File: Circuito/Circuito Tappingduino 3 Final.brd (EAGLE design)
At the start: 90.5 x 69 mm, 67 parts, among them IC1 LM324N

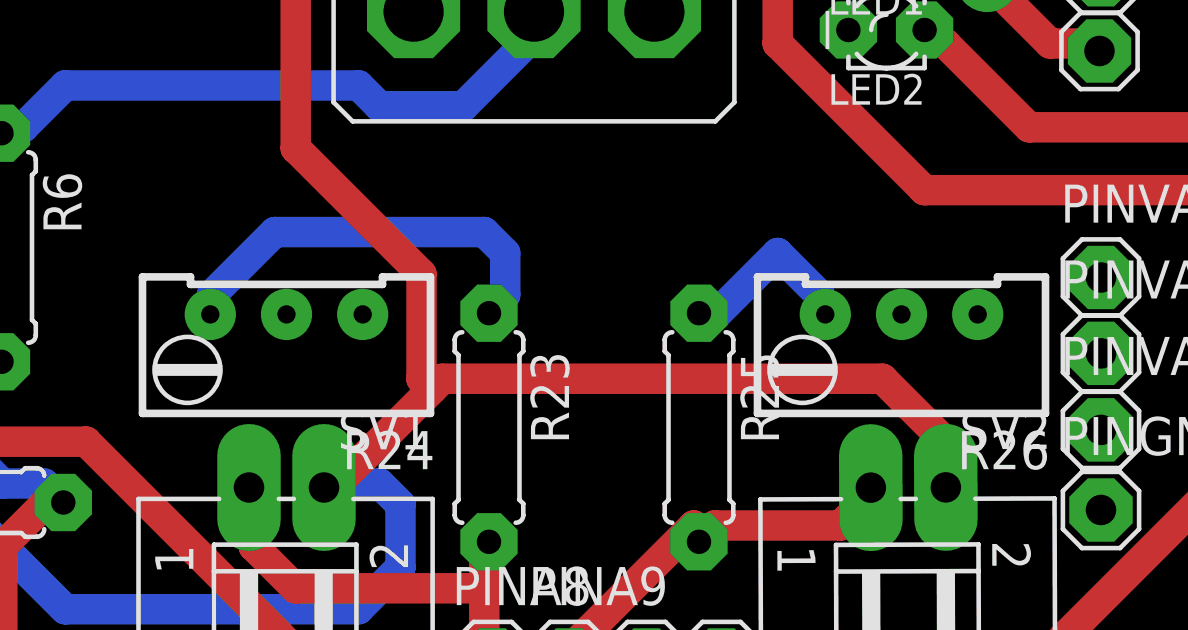
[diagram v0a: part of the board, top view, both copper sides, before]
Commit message: Version final del circuito
Lo vuelvo a subir porque no estaba segura de haber guardado el archivo de eagle que tiene ya las vias adicionales en la resistencia variable que tenia los pads muy chicos.
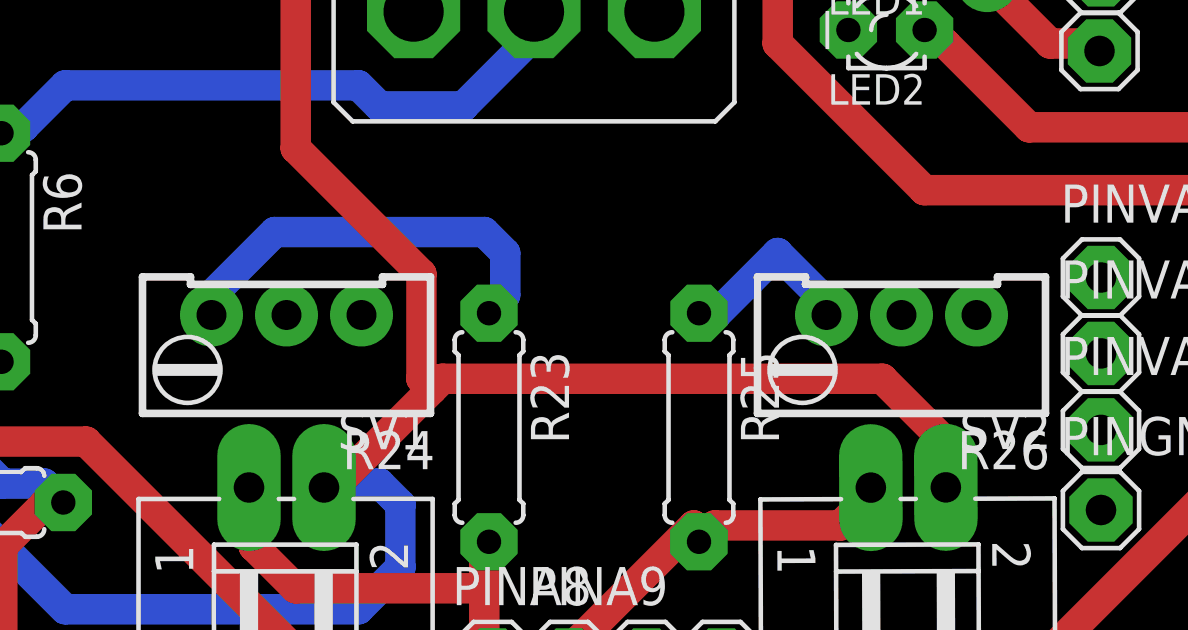
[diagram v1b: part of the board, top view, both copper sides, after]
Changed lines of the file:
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@@
 <grid distance="0.25" unitdist="mm" unit="mm" style="lines" multiple="1" display="yes" altdistance="0.025" altunitdist="inch" altunit="inch"/>
 <layers>
-<layer number="1" name="Top" color="4" fill="1" visible="yes" active="yes"/>
+<layer number="1" name="Top" color="4" fill="1" visible="no" active="yes"/>
 <layer number="2" name="Route2" color="1" fill="3" visible="no" active="no"/>
 <layer number="3" name="Route3" color="4" fill="3" visible="no" active="no"/>
@@
 <layer number="17" name="Pads" color="2" fill="1" visible="yes" active="yes"/>
 <layer number="18" name="Vias" color="2" fill="1" visible="yes" active="yes"/>
-<layer number="19" name="Unrouted" color="6" fill="1" visible="yes" active="yes"/>
-<layer number="20" name="Dimension" color="15" fill="1" visible="yes" active="yes"/>
-<layer number="21" name="tPlace" color="7" fill="1" visible="yes" active="yes"/>
-<layer number="22" name="bPlace" color="7" fill="1" visible="yes" active="yes"/>
-<layer number="23" name="tOrigins" color="15" fill="1" visible="yes" active="yes"/>
-<layer number="24" name="bOrigins" color="15" fill="1" visible="yes" active="yes"/>
-<layer number="25" name="tNames" color="7" fill="1" visible="yes" active="yes"/>
-<layer number="26" name="bNames" color="7" fill="1" visible="yes" active="yes"/>
-<layer number="27" name="tValues" color="7" fill="1" visible="yes" active="yes"/>
-<layer number="28" name="bValues" color="7" fill="1" visible="yes" active="yes"/>
+<layer number="19" name="Unrouted" color="6" fill="1" visible="no" active="yes"/>
+<layer number="20" name="Dimension" color="15" fill="1" visible="no" active="yes"/>
+<layer number="21" name="tPlace" color="7" fill="1" visible="no" active="yes"/>
+<layer number="22" name="bPlace" color="7" fill="1" visible="no" active="yes"/>
+<layer number="23" name="tOrigins" color="15" fill="1" visible="no" active="yes"/>
+<layer number="24" name="bOrigins" color="15" fill="1" visible="no" active="yes"/>
+<layer number="25" name="tNames" color="7" fill="1" visible="no" active="yes"/>
+<layer number="26" name="bNames" color="7" fill="1" visible="no" active="yes"/>
+<layer number="27" name="tValues" color="7" fill="1" visible="no" active="yes"/>
+<layer number="28" name="bValues" color="7" fill="1" visible="no" active="yes"/>
 <layer number="29" name="tStop" color="7" fill="3" visible="no" active="yes"/>
 <layer number="30" name="bStop" color="7" fill="6" visible="no" active="yes"/>
@@
 <layer number="39" name="tKeepout" color="4" fill="11" visible="no" active="yes"/>
 <layer number="40" name="bKeepout" color="1" fill="11" visible="no" active="yes"/>
-<layer number="41" name="tRestrict" color="4" fill="10" visible="yes" active="yes"/>
-<layer number="42" name="bRestrict" color="1" fill="10" visible="yes" active="yes"/>
-<layer number="43" name="vRestrict" color="2" fill="10" visible="yes" active="yes"/>
+<layer number="41" name="tRestrict" color="4" fill="10" visible="no" active="yes"/>
+<layer number="42" name="bRestrict" color="1" fill="10" visible="no" active="yes"/>
+<layer number="43" name="vRestrict" color="2" fill="10" visible="no" active="yes"/>
 <layer number="44" name="Drills" color="7" fill="1" visible="no" active="yes"/>
 <layer number="45" name="Holes" color="7" fill="1" visible="no" active="yes"/>
@@
 <vertex x="103.5" y="65.25"/>
 </polygon>
+<wire x1="93.9" y1="7.5" x2="87.25" y2="14.02" width="0" layer="19" extent="1-1"/>
+<wire x1="66.75" y1="14.02" x2="52.25" y2="27.44" width="0" layer="19" extent="1-1"/>
 </signal>
 <signal name="N$1">
@@
 <wire x1="58.674" y1="8.382" x2="59.31" y2="7.75" width="1.016" layer="16"/>
 </signal>
+<signal name="N$12">
+<via x="64.25" y="14" extent="1-16" drill="1"/>
+</signal>
+<signal name="N$33">
+<via x="66.75" y="14" extent="1-16" drill="1"/>
+</signal>
+<signal name="N$35">
+<via x="69.25" y="14" extent="1-16" drill="1"/>
+</signal>
+<signal name="N$36">
+<via x="84.75" y="14" extent="1-16" drill="1"/>
+</signal>
+<signal name="N$38">
+<via x="87.25" y="14" extent="1-16" drill="1"/>
+</signal>
+<signal name="N$39">
+<via x="89.75" y="14" extent="1-16" drill="1"/>
+</signal>
 </signals>
